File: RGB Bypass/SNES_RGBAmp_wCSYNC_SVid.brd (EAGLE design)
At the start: 23.5 x 20.6 mm, 31 parts, among them J3 SNES_MULTIAV_RGBC_ONLY, U1 THS7374

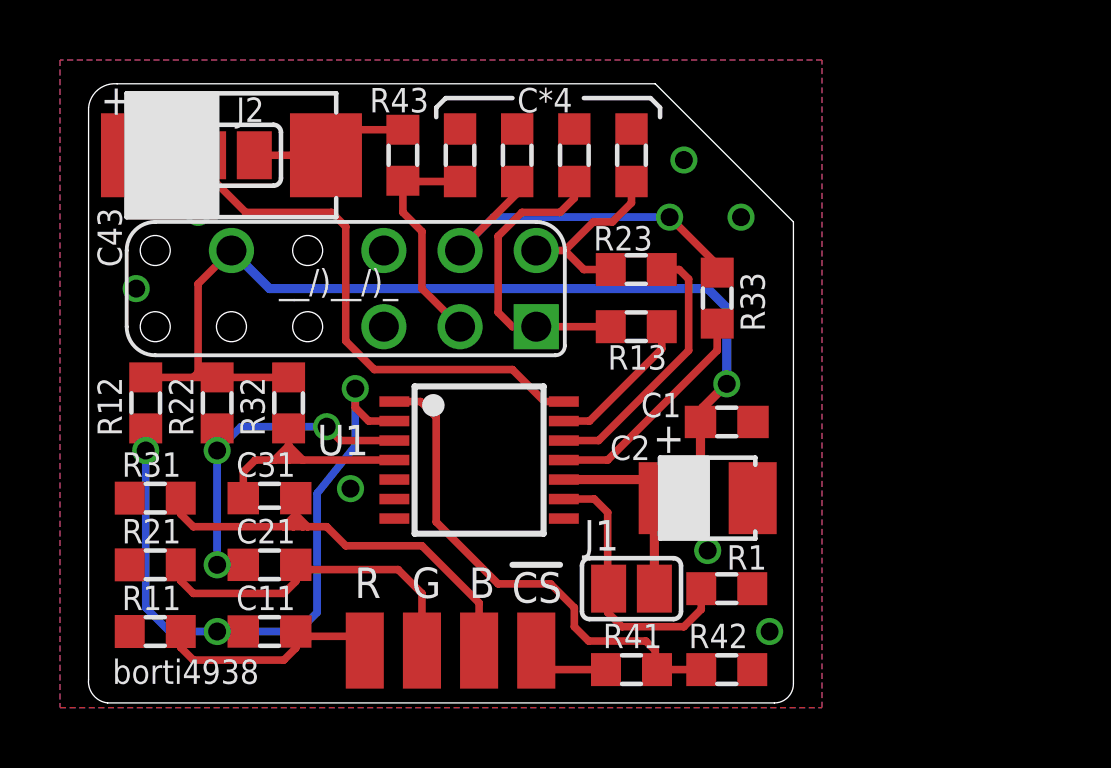
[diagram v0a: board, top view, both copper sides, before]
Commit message: go to version 4.1
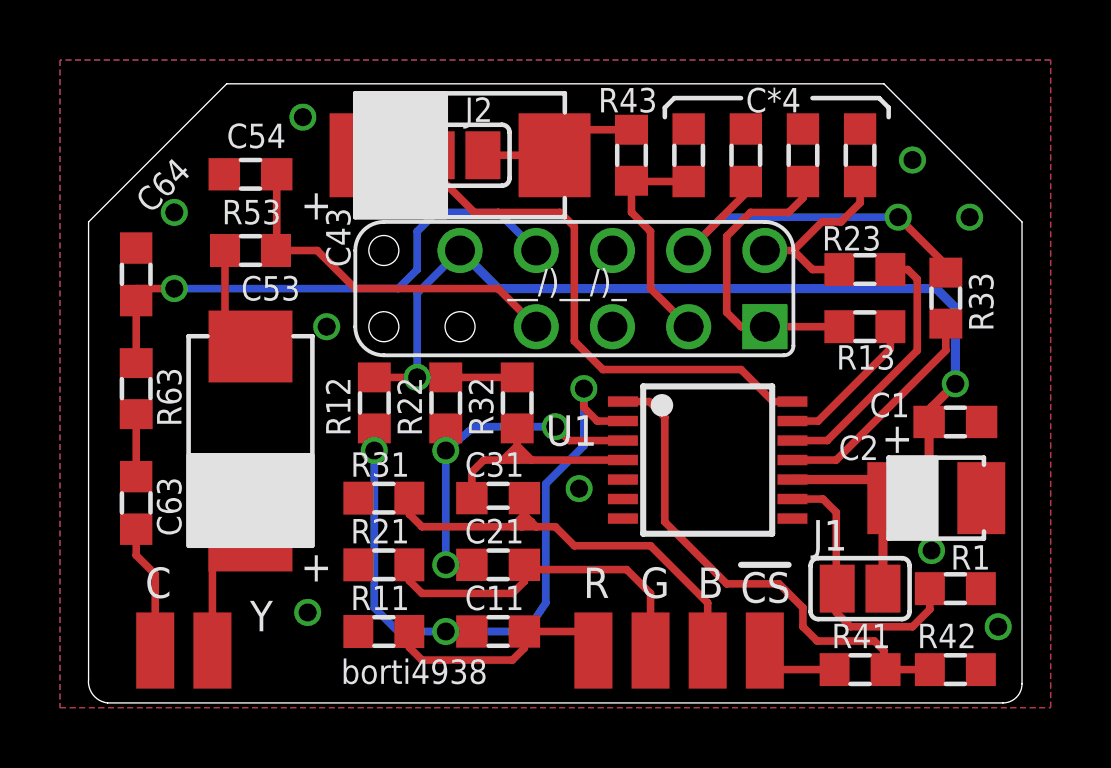
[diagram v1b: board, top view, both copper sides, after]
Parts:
- removed J3: SNES_MULTIAV_RGBC_ONLY, snes_div:SNES_MULTIAV_RGBC_ONLY
- added C, Y: (no value), wirepad:SMD1,27-2,54
- added C53: 330u, rcl:SMC_D
- added C54, C64: 47p, rcl:C0603K
- added C63: 100n, rcl:C0603K
- added R53, R63: (no value), rcl:R0603
- added U$1: SNES_MULTIAV_RGBSYC, snes_div:SNES_MULTIAV_RGBSYC
- moved C14 7.62 mm to (24.8, 18.4)
- moved C2 7.62 mm to (29.2, 6.99)
- moved C24 7.62 mm to (26.7, 18.4)
- moved C43 7.62 mm to (13.3, 18.4)
- moved CS 7.62 mm to (23.5, 1.91)
- moved J1 7.62 mm to (26.7, 3.97)
- moved J2 7.62 mm to (13.3, 18.4)
- moved R 7.62 mm to (17.8, 1.91)
- moved R13 7.62 mm to (26.8, 12.7)
- moved R22 7.62 mm to (12.9, 10.2)
- moved R23 7.62 mm to (26.8, 14.6)
- moved R33 7.62 mm to (29.5, 13.7)
- moved R41 7.62 mm to (26.7, 1.27)
- moved R43 7.62 mm to (19.1, 18.4)
- moved C11 7.62 mm to (14.6, 2.54)
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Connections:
- new net N$12: C53.+, Y.1
- new net N$13: C.1, C63.2
- new net N$20: C53.-, R53.1
- new net N$21: C54.2, R53.2, U$1.Y
- new net N$22: C64.2, R63.2, U$1.C
- new net N$23: C63.1, R63.1
- net GND: now also C54.1, C64.1, U$1.P$5, U$1.P$6; no longer J3.P$5, J3.P$6
- net N$4: now also U$1.P$3; no longer J3.P$3
- net N$5: now also U$1.P$1; no longer J3.P$1
- net N$6: now also U$1.P$2; no longer J3.P$2
- net N$9: now also U$1.P$4; no longer J3.P$4
- net VCC: now also U$1.P$10; no longer J3.P$10
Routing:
- net N$22: track 0.00 -> 18.1 mm, vias 0 -> 1
- net N$21: track 0.00 -> 12.3 mm
- net N$12: track 0.00 -> 5.00 mm
- net N$13: track 0.00 -> 4.31 mm
- net N$20: track 0.00 -> 3.55 mm
- net N$23: track 0.00 -> 2.09 mm
- net N$16: track 16.0 -> 15.4 mm
- net GND: track 0.00 -> 0.11 mm, vias 7 -> 9
- net VCC: track 41.7 -> 41.8 mm, vias 1 -> 2
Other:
- board size 23.5 x 20.6 mm -> 31.1 x 20.6 mm
- board text added: "C53"
- board text added: "C54"
- board text added: "C63"
- board text added: "C64"
- board text added: "R53"
- board text added: "R63"
- board text added: "SNES-Mini/Jr. RGB Amp V4.1a + S-Video"
- board text removed: "SNES RGB Amp V4.1a"

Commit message: Change resistor values
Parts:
- R12, R22, R32: value 3M6 -> 5M1
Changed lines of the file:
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@@
 <?xml version="1.0" encoding="utf-8"?>
 <!DOCTYPE eagle SYSTEM "eagle.dtd">
-<eagle version="6.4">
+<eagle version="7.7.0">
 <drawing>
 <settings>
@@
 <pass name="Default">
 <param name="RoutingGrid" value="50mil"/>
+<param name="AutoGrid" value="1"/>
+<param name="Efforts" value="0"/>
+<param name="TopRouterVariant" value="1"/>
 <param name="tpViaShape" value="round"/>
 <param name="PrefDir.1" value="|"/>
@@
 <attribute name="VALUE" x="10.16" y="5.08" size="1.27" layer="27"/>
 </element>
-<element name="R12" library="rcl" package="R0603" value="3M6" x="10.4775" y="10.16" smashed="yes" rot="R90"/>
-<element name="R22" library="rcl" package="R0603" value="3M6" x="12.85875" y="10.16" smashed="yes" rot="R90"/>
-<element name="R32" library="rcl" package="R0603" value="3M6" x="15.24" y="10.16" smashed="yes" rot="R90"/>
+<element name="R12" library="rcl" package="R0603" value="5M1" x="10.4775" y="10.16" smashed="yes" rot="R90"/>
+<element name="R22" library="rcl" package="R0603" value="5M1" x="12.85875" y="10.16" smashed="yes" rot="R90"/>
+<element name="R32" library="rcl" package="R0603" value="5M1" x="15.24" y="10.16" smashed="yes" rot="R90"/>
 <element name="R13" library="rcl" package="R0603" value="" x="26.82875" y="12.7" smashed="yes">
 <attribute name="VALUE" x="26.19375" y="10.795" size="1.27" layer="27"/>
